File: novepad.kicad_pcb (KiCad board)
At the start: 4 copper layers, 99 x 59.5 mm, 27 parts, among them J101 NOVENA_LCD_CONN, J102 LP097QX1_CONN, J401 MOLEX_502250-8037, J402 MOLEX_502250-8037, U301 IT6251, U401 FT5816LPC

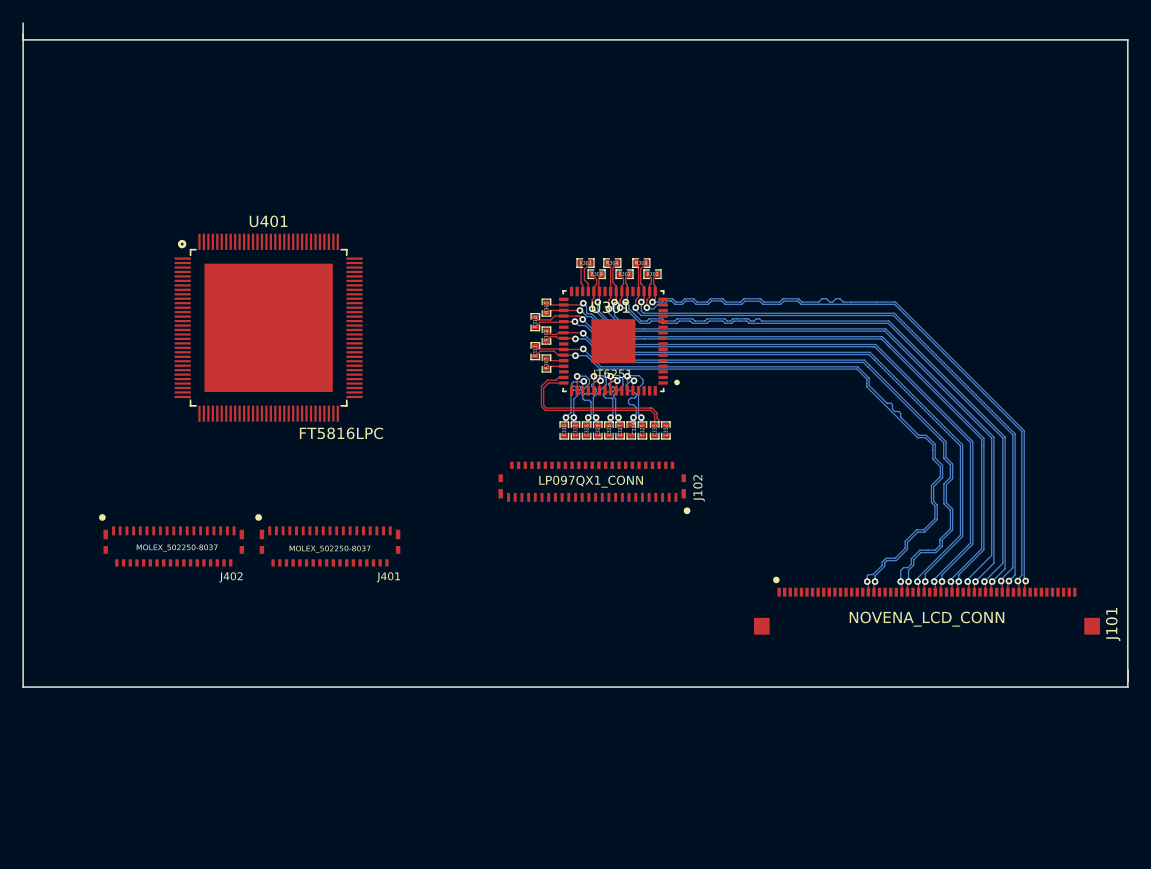
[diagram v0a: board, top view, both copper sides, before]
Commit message: Super-zealous length matching version
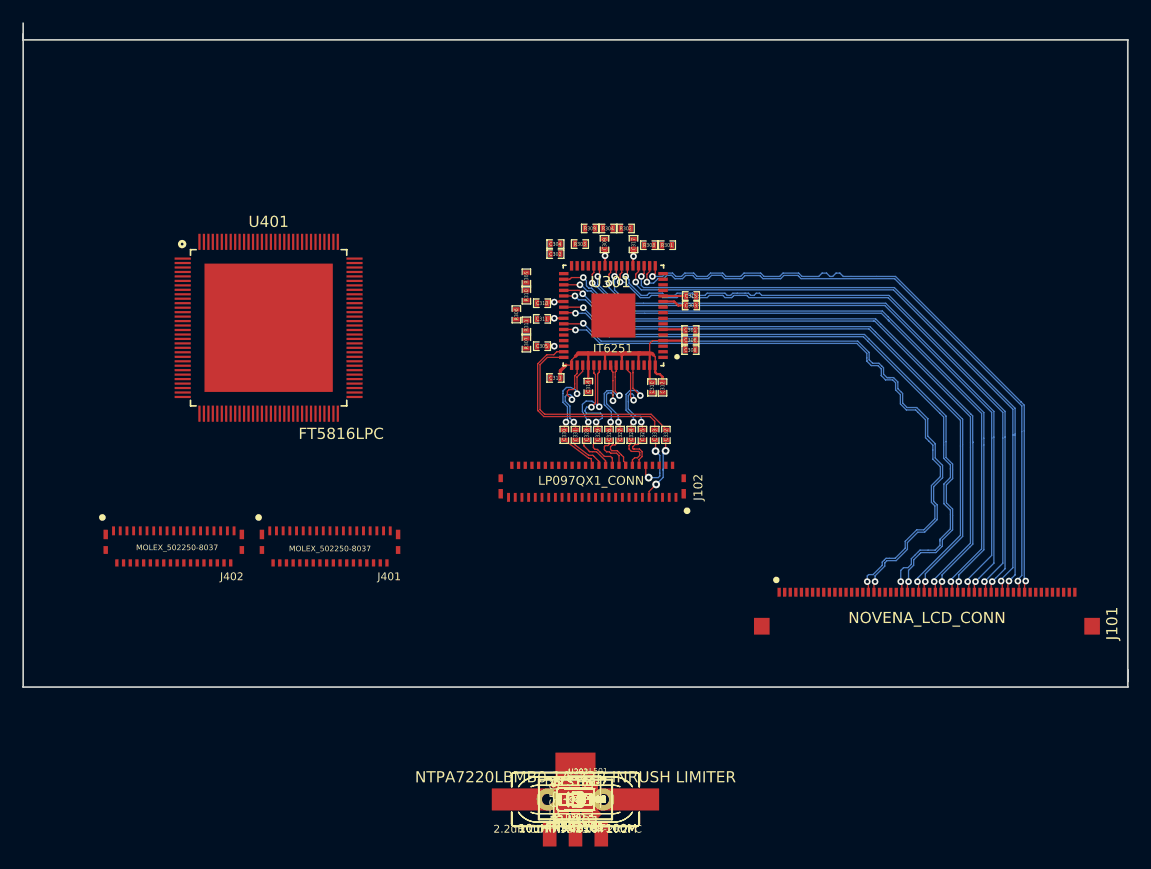
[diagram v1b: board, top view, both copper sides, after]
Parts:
- added C201, C203, C207, C208: 4.7uF 25V, FT:1206, F.Cu at (137.5, 165.1)
- added C202, C204: 1uF 25V, FT:1206, F.Cu at (137.5, 165.1)
- added C205, C206: 100nF, FT:C0402, F.Cu at (137.5, 165.1)
- added C301: 100nF 25V X5R, SMD_Packages:SMD-0402_c, F.Cu at (147.8, 123.0)
- added C302: 100nF 25V X5R, SMD_Packages:SMD-0402_c, F.Cu at (135.7, 116.2)
- added C303: 100nF 25V X5R, SMD_Packages:SMD-0402_c, F.Cu at (147.8, 120.8)
- added C304: 1nF 25V X5R, SMD_Packages:SMD-0402_c, F.Cu at (135.7, 115.3)
- added C305: 100nF 25V X5R, SMD_Packages:SMD-0402_c, F.Cu at (134.5, 124.5)
- added C306: 100nF 25V X5R, SMD_Packages:SMD-0402_c, F.Cu at (147.8, 123.9)
- added C308: 1nF 25V X5R, SMD_Packages:SMD-0402_c, F.Cu at (147.8, 124.8)
- added C309: 100nF 25V X5R, SMD_Packages:SMD-0402_c, F.Cu at (140.1, 115.3)
- added C310: 100nF 25V X5R, SMD_Packages:SMD-0402_c, F.Cu at (144.3, 128.2)
- added C311: 100nF 25V X5R, SMD_Packages:SMD-0402_c, F.Cu at (134.5, 122.0)
- added C312: 1nF 25V X5R, SMD_Packages:SMD-0402_c, F.Cu at (145.3, 128.2)
- added C313: 100nF 25V X5R, SMD_Packages:SMD-0402_c, F.Cu at (135.7, 127.3)
- added C314: 100nF 25V X5R, SMD_Packages:SMD-0402_c, F.Cu at (138.7, 128.1)
- added C315: 1uF 25V X5R, SMD_Packages:SMD-0402_c, F.Cu at (147.8, 120.0)
- added C317: 100nF 25V X5R, SMD_Packages:SMD-0402_c, F.Cu at (142.7, 115.3)
- added C318: 100nF 25V X5R, SMD_Packages:SMD-0402_c, F.Cu at (134.5, 120.6)
- added C319, C323: 100nF 25V X5R, SMD_Packages:SMD-0402_c, F.Cu at (137.5, 165.1)
- added C321, C322, C405, C408: 27pF, FT:0603, F.Cu at (137.5, 165.1)
- added C401: 10uF 10V, FT:1206, F.Cu at (137.5, 165.1)
- added C402: 100nF 10V, SMD_Packages:SMD-0402_c, F.Cu at (137.5, 165.1)
- added C403, C404, C406, C407, C409: 1uF 10V, FT:1206, F.Cu at (137.5, 165.1)
- added C501, C502, C503, C504, C505, C506: 10uF 10V X5R, FT:1206, F.Cu at (137.5, 165.1)
- added D201, D202, D501: DFLS160-7, novepad:POWERDI123_DIODE, F.Cu at (137.5, 165.1)
- added L201, L202: 10uH NR4018T100M, novepad:NR4018_IND, F.Cu at (137.5, 165.1)
- added L401, L502, L503: BLM18KG121, FT:0603, F.Cu at (137.5, 165.1)
- added L501: 2.2uH CDRH3D23NP-2R2PC, novepad:CDRH3D23_IND, F.Cu at (137.5, 165.1)
- added R201, R402, R407: 0R DNP, FT:0603, F.Cu at (137.5, 165.1)
- added R202, R203: 51R, FT:0603, F.Cu at (137.5, 165.1)
- added R204, R205: 68K 1%, FT:0603, F.Cu at (137.5, 165.1)
- added R312, R314, R401, R406: 10K, FT:0603, F.Cu at (137.5, 165.1)
- added R313, R405: 10K DNP, FT:0603, F.Cu at (137.5, 165.1)
- added R315, R409: 1M, FT:0603, F.Cu at (137.5, 165.1)
- added R316: 820R 1%, FT:0603, F.Cu at (137.5, 165.1)
- added R317: 33R 1%, FT:0603, F.Cu at (137.5, 165.1)
- added R318: 100K DNP, FT:0603, F.Cu at (137.5, 165.1)
- added R319: 100K, FT:0603, F.Cu at (137.5, 165.1)
- added R403, R404: 22R, FT:0603, F.Cu at (137.5, 165.1)
- added R408: 10R, FT:0603, F.Cu at (137.5, 165.1)
- added R501: 10K 1%, FT:0603, F.Cu at (137.5, 165.1)
- added R502: 20K 1%, FT:0603, F.Cu at (137.5, 165.1)
- added REG501: NCP1117ST18T3G DNP, FT:SOT223, F.Cu at (137.5, 165.1)
- added REG502: LMR10510YSD, novepad:WSON6, F.Cu at (137.5, 165.1)
- added SJ101, SJ102, SJ501: SJ, FT:SJ_SHORTED, F.Cu at (137.5, 165.1)
- added TH201: NTPA7220LBMB0 1A 22R INRUSH LIMITER, novepad:PTH_2HOLE_5MM, F.Cu at (137.5, 165.1)
- added TP201, TP202, TP203, TP204, TP205, TP206, TP301, TP302, TP303, TP304, TP305, TP306, TP401, TP402, TP403, TP404, TP405, TP406, TP407, TP408, TP409, TP410, TP411, TP412, TP413, TP414, TP415, TP416, TP501, TP502: CONN_1, novepad:SMD_TEST_POINT, F.Cu at (137.5, 165.1)
- added U201, U202: TPS61181, novepad:QFN50P300X300X80-17N, F.Cu at (137.5, 165.1)
- added X301: 27MHz 50ppm, 8-18pF, ESR < 80ohm, FT:HC49UP, F.Cu at (137.5, 165.1)
- added X401: 12MHz 18pF, FT:HC49UP, F.Cu at (137.5, 165.1)
- moved R309 4.14 mm to (138.8, 113.9)
- moved R302 4.10 mm to (142.0, 113.9)
- moved R306 3.30 mm to (132.2, 121.6)
- moved R305 3.24 mm to (133.1, 118.3)
- moved R304 3.13 mm to (140.4, 113.9)
- moved R301 2.91 mm to (145.7, 115.4)
- moved R307 2.55 mm to (133.1, 124.2)
- moved R310 2.53 mm to (133.1, 119.9)
- moved R311 2.44 mm to (133.1, 122.6)
- moved U301 2.30 mm to (140.9, 121.7)
- moved R303 1.77 mm to (137.9, 115.3)
- moved R308 1.75 mm to (144.1, 115.4)
- moved C324 0.40 mm to (142.5, 132.4)
- moved C325 0.40 mm to (143.5, 132.4)
- moved C326 0.40 mm to (140.5, 132.4)
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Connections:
- U401 pad 1: /Capacitive Touch (Optional)/TX8 -> /Capacitive Touch (Optional)/TX33
- U401 pad 10: /Capacitive Touch (Optional)/TX17 -> /Capacitive Touch (Optional)/TX24
- U401 pad 100: /Capacitive Touch (Optional)/RX5 -> /Capacitive Touch (Optional)/RX26
- U401 pad 101: /Capacitive Touch (Optional)/RX6 -> /Capacitive Touch (Optional)/RX25
- U401 pad 102: /Capacitive Touch (Optional)/RX7 -> /Capacitive Touch (Optional)/RX24
- U401 pad 103: /Capacitive Touch (Optional)/RX8 -> /Capacitive Touch (Optional)/RX23
- U401 pad 104: /Capacitive Touch (Optional)/RX9 -> /Capacitive Touch (Optional)/RX22
- U401 pad 105: /Capacitive Touch (Optional)/RX10 -> /Capacitive Touch (Optional)/RX21
- U401 pad 106: /Capacitive Touch (Optional)/RX11 -> /Capacitive Touch (Optional)/RX20
- U401 pad 107: /Capacitive Touch (Optional)/RX12 -> /Capacitive Touch (Optional)/RX19
- U401 pad 108: /Capacitive Touch (Optional)/RX13 -> /Capacitive Touch (Optional)/RX18
- U401 pad 109: /Capacitive Touch (Optional)/RX14 -> /Capacitive Touch (Optional)/RX17
- U401 pad 11: /Capacitive Touch (Optional)/TX18 -> /Capacitive Touch (Optional)/TX23
- U401 pad 110: /Capacitive Touch (Optional)/RX15 -> /Capacitive Touch (Optional)/RX16
- U401 pad 111: /Capacitive Touch (Optional)/RX16 -> /Capacitive Touch (Optional)/RX15
- U401 pad 112: /Capacitive Touch (Optional)/RX17 -> /Capacitive Touch (Optional)/RX14
- U401 pad 113: /Capacitive Touch (Optional)/RX18 -> /Capacitive Touch (Optional)/RX13
- U401 pad 119: /Capacitive Touch (Optional)/TX1 -> /Capacitive Touch (Optional)/TX40
- U401 pad 12: /Capacitive Touch (Optional)/TX19 -> /Capacitive Touch (Optional)/TX22
- U401 pad 120: /Capacitive Touch (Optional)/TX2 -> /Capacitive Touch (Optional)/TX39
- U401 pad 121: /Capacitive Touch (Optional)/TX3 -> /Capacitive Touch (Optional)/TX38
- U401 pad 122: /Capacitive Touch (Optional)/TX4 -> /Capacitive Touch (Optional)/TX37
- U401 pad 123: /Capacitive Touch (Optional)/TX5 -> /Capacitive Touch (Optional)/TX36
- U401 pad 124: /Capacitive Touch (Optional)/TX6 -> /Capacitive Touch (Optional)/TX35
- U401 pad 125: /Capacitive Touch (Optional)/TX7 -> /Capacitive Touch (Optional)/TX34
- U401 pad 13: /Capacitive Touch (Optional)/TX20 -> /Capacitive Touch (Optional)/TX21
- U401 pad 14: /Capacitive Touch (Optional)/TX21 -> /Capacitive Touch (Optional)/TX20
- U401 pad 15: /Capacitive Touch (Optional)/TX22 -> /Capacitive Touch (Optional)/TX19
- U401 pad 16: /Capacitive Touch (Optional)/TX23 -> /Capacitive Touch (Optional)/TX18
- U401 pad 2: /Capacitive Touch (Optional)/TX9 -> /Capacitive Touch (Optional)/TX32
- U401 pad 20: /Capacitive Touch (Optional)/TX24 -> /Capacitive Touch (Optional)/TX17
- U401 pad 21: /Capacitive Touch (Optional)/TX25 -> /Capacitive Touch (Optional)/TX16
- U401 pad 22: /Capacitive Touch (Optional)/TX26 -> /Capacitive Touch (Optional)/TX15
- U401 pad 23: /Capacitive Touch (Optional)/TX27 -> /Capacitive Touch (Optional)/TX14
- U401 pad 24: /Capacitive Touch (Optional)/TX28 -> /Capacitive Touch (Optional)/TX13
- U401 pad 25: /Capacitive Touch (Optional)/TX29 -> /Capacitive Touch (Optional)/TX12
- U401 pad 26: /Capacitive Touch (Optional)/TX30 -> /Capacitive Touch (Optional)/TX11
- U401 pad 27: /Capacitive Touch (Optional)/TX31 -> /Capacitive Touch (Optional)/TX10
- U401 pad 28: /Capacitive Touch (Optional)/TX32 -> /Capacitive Touch (Optional)/TX9
- U401 pad 29: /Capacitive Touch (Optional)/TX33 -> /Capacitive Touch (Optional)/TX8
- U401 pad 3: /Capacitive Touch (Optional)/TX10 -> /Capacitive Touch (Optional)/TX31
- U401 pad 30: /Capacitive Touch (Optional)/TX34 -> /Capacitive Touch (Optional)/TX7
- U401 pad 31: /Capacitive Touch (Optional)/TX35 -> /Capacitive Touch (Optional)/TX6
- U401 pad 32: /Capacitive Touch (Optional)/TX36 -> /Capacitive Touch (Optional)/TX5
- U401 pad 33: /Capacitive Touch (Optional)/TX37 -> /Capacitive Touch (Optional)/TX4
- U401 pad 34: /Capacitive Touch (Optional)/TX38 -> /Capacitive Touch (Optional)/TX3
- U401 pad 35: /Capacitive Touch (Optional)/TX39 -> /Capacitive Touch (Optional)/TX2
- U401 pad 36: /Capacitive Touch (Optional)/TX40 -> /Capacitive Touch (Optional)/TX1
- U401 pad 4: /Capacitive Touch (Optional)/TX11 -> /Capacitive Touch (Optional)/TX30
- U401 pad 5: /Capacitive Touch (Optional)/TX12 -> /Capacitive Touch (Optional)/TX29
- U401 pad 54: /Capacitive Touch (Optional)/RX30 -> /Capacitive Touch (Optional)/RX1
- U401 pad 55: /Capacitive Touch (Optional)/RX29 -> /Capacitive Touch (Optional)/RX2
- U401 pad 56: /Capacitive Touch (Optional)/RX28 -> /Capacitive Touch (Optional)/RX3
- U401 pad 57: /Capacitive Touch (Optional)/RX27 -> /Capacitive Touch (Optional)/RX4
- U401 pad 58: /Capacitive Touch (Optional)/RX26 -> /Capacitive Touch (Optional)/RX5
- U401 pad 59: /Capacitive Touch (Optional)/RX25 -> /Capacitive Touch (Optional)/RX6
- U401 pad 6: /Capacitive Touch (Optional)/TX13 -> /Capacitive Touch (Optional)/TX28
- U401 pad 60: /Capacitive Touch (Optional)/RX24 -> /Capacitive Touch (Optional)/RX7
- U401 pad 61: /Capacitive Touch (Optional)/RX23 -> /Capacitive Touch (Optional)/RX8
- U401 pad 62: /Capacitive Touch (Optional)/RX22 -> /Capacitive Touch (Optional)/RX9
- U401 pad 63: /Capacitive Touch (Optional)/RX21 -> /Capacitive Touch (Optional)/RX10
- U401 pad 64: /Capacitive Touch (Optional)/RX20 -> /Capacitive Touch (Optional)/RX11
- U401 pad 65: /Capacitive Touch (Optional)/RX19 -> /Capacitive Touch (Optional)/RX12
- U401 pad 7: /Capacitive Touch (Optional)/TX14 -> /Capacitive Touch (Optional)/TX27
- U401 pad 8: /Capacitive Touch (Optional)/TX15 -> /Capacitive Touch (Optional)/TX26
- U401 pad 9: /Capacitive Touch (Optional)/TX16 -> /Capacitive Touch (Optional)/TX25
- U401 pad 96: /Capacitive Touch (Optional)/RX1 -> /Capacitive Touch (Optional)/RX30
- U401 pad 97: /Capacitive Touch (Optional)/RX2 -> /Capacitive Touch (Optional)/RX29
- U401 pad 98: /Capacitive Touch (Optional)/RX3 -> /Capacitive Touch (Optional)/RX28
- U401 pad 99: /Capacitive Touch (Optional)/RX4 -> /Capacitive Touch (Optional)/RX27
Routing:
- net +1.8VA: track 0.00 -> 32.3 mm, vias 0 -> 2
- net /LVDS to eDP Conversion/eDP_AUX_P: track 0.00 -> 5.85 mm, vias 0 -> 2
- net /LVDS to eDP Conversion/eDP_AUX_N: track 0.00 -> 5.70 mm, vias 0 -> 2
- net +3.3V: track 0.00 -> 5.13 mm, vias 0 -> 2
- net +1.8V: track 0.00 -> 4.87 mm, vias 0 -> 1
- net /LVDS to eDP Conversion/eDP_LANE1_N: track 0.00 -> 3.62 mm
- net /LVDS to eDP Conversion/eDP_LANE3_N: track 0.00 -> 3.61 mm
- net /LVDS to eDP Conversion/eDP_LANE2_N: track 0.00 -> 3.59 mm
- net /LVDS to eDP Conversion/eDP_LANE0_N: track 0.00 -> 3.58 mm
- net /LVDS to eDP Conversion/eDP_LANE1_P: track 0.00 -> 3.57 mm
- net /LVDS to eDP Conversion/eDP_LANE0_P: track 0.00 -> 3.56 mm
- net /LVDS to eDP Conversion/eDP_LANE3_P: track 0.00 -> 3.55 mm
- net /LVDS to eDP Conversion/eDP_LANE2_P: track 0.00 -> 3.55 mm
- net /LVDS to eDP Conversion/RXNE1: track 2.92 -> 0.00 mm
- net /LVDS to eDP Conversion/AUX_P: track 15.5 -> 18.4 mm
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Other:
- net class Power: clearance 0.3 -> 0.2
- net class eDP_AUX_OUT_LM0.5 added: clearance 0.2, trace_width 0.2, via_dia 0.7, via_drill 0.4
